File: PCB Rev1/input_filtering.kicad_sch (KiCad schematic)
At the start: 13 parts, among them U1 LMR43620MSC5-Q1RPE

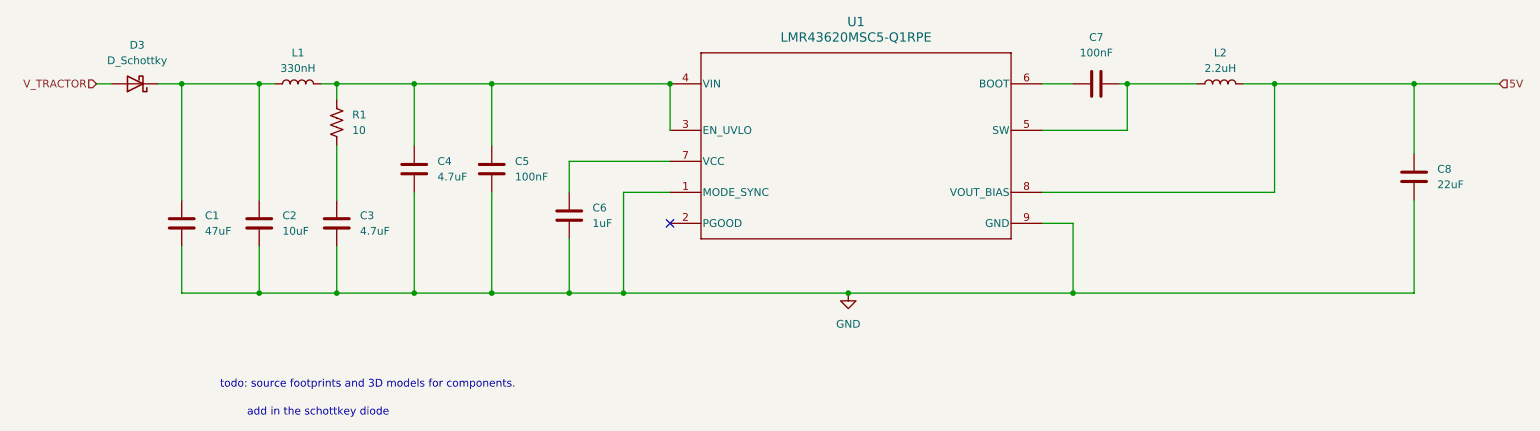
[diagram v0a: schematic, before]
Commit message: added PCB rev2!
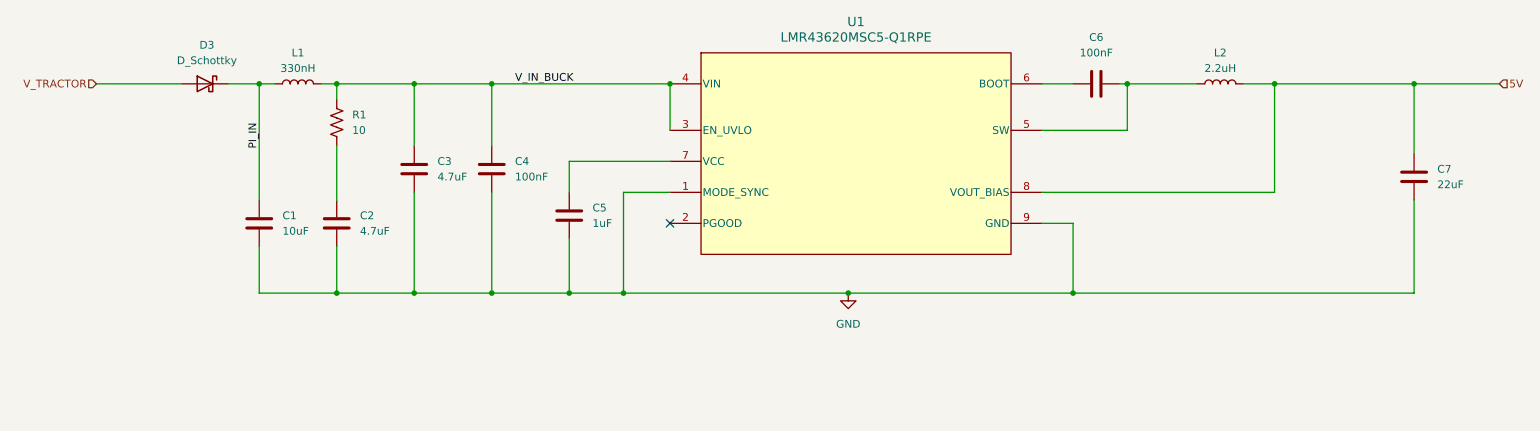
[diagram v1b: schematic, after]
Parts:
- removed C1: 47uF, symbol Device:C
- C1: renamed from C2; footprint (none) -> footprints:CAPC3216X190N; Part # (none) -> CGA5L1X7R1H106K160AE
- C2: renamed from C3; footprint (none) -> footprints:CAPC2012X150N; Part # (none) -> CGA4J1X7R1H475K125AC
- C3: renamed from C4; footprint (none) -> footprints:CAPC2012X150N; Part # (none) -> CGA4J1X7R1H475K125AC
- C4: renamed from C5; footprint (none) -> footprints:CAPC2012X94N; Part # (none) -> 08055C104K4Z2A
- C5: renamed from C6; footprint (none) -> Capacitor_SMD:C_0805_2012Metric; Part # (none) -> UMK212B7105KGHT
- C6: renamed from C7; footprint (none) -> footprints:CAPC1005X55N; Part # (none) -> LMK105B7104KVHF
- C7: renamed from C8; footprint (none) -> footprints:CAPC3216X190N; Part # (none) -> LMJ316BB7226KLHT
- D3: footprint (none) -> footprints:CR_SMP_DO-220AA_VIS; Part # (none) -> SS2PH5HM3-84A
- L1: footprint (none) -> footprints:WE-MAPI_2510; Part # (none) -> 744383230033
- R1: footprint (none) -> footprints:RES_ERJ3EKF10R0V; Part # (none) -> ERJ-3EKF10R0V
- U1: Part # (none) -> LMR43620MSC5-Q1RPE
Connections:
- net V_TRACTOR: now also D3.1 (K); no longer D3.2 (A)
- net V_IN_BUCK: now reaches C3.1, C4.1, L1.2, R1.1, U1.3 (EN_UVLO), U1.4 (VIN)
- net PI_IN: now reaches C1.1, L1.1
- net PI_IN: now also D3.2 (A); no longer D3.1 (K)
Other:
- note removed: "add in the schottkey diode"
- note removed: "todo: source footprints and 3D models for components."
- moved on the sheet: D3
